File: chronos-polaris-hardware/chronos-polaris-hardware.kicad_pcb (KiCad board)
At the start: 2 copper layers, 65 parts, among them J1 Conn_01x03_Pin, J2 Conn_01x03_Pin, J3 Conn_01x03_Pin, J4 Conn_01x03_Pin, J5 Conn_01x03_Pin, J6 Conn_01x04, J7 Conn_01x04, J8 Conn_01x02, J9 691417320006S, Q1 US6K4TR, U1 TLV62130RGTR, U10 MSK12C02-HB, U11 TPS62172DSGR, U14 FC-B1010RGBT-HG, U2 ESP32-S2-SOLO-2-N4, U3 BMI088, U4 TYPE-C_14PLC-H10_0, U5 TF_PUSH, U6 TPS629206DRLR, U9 BMP280

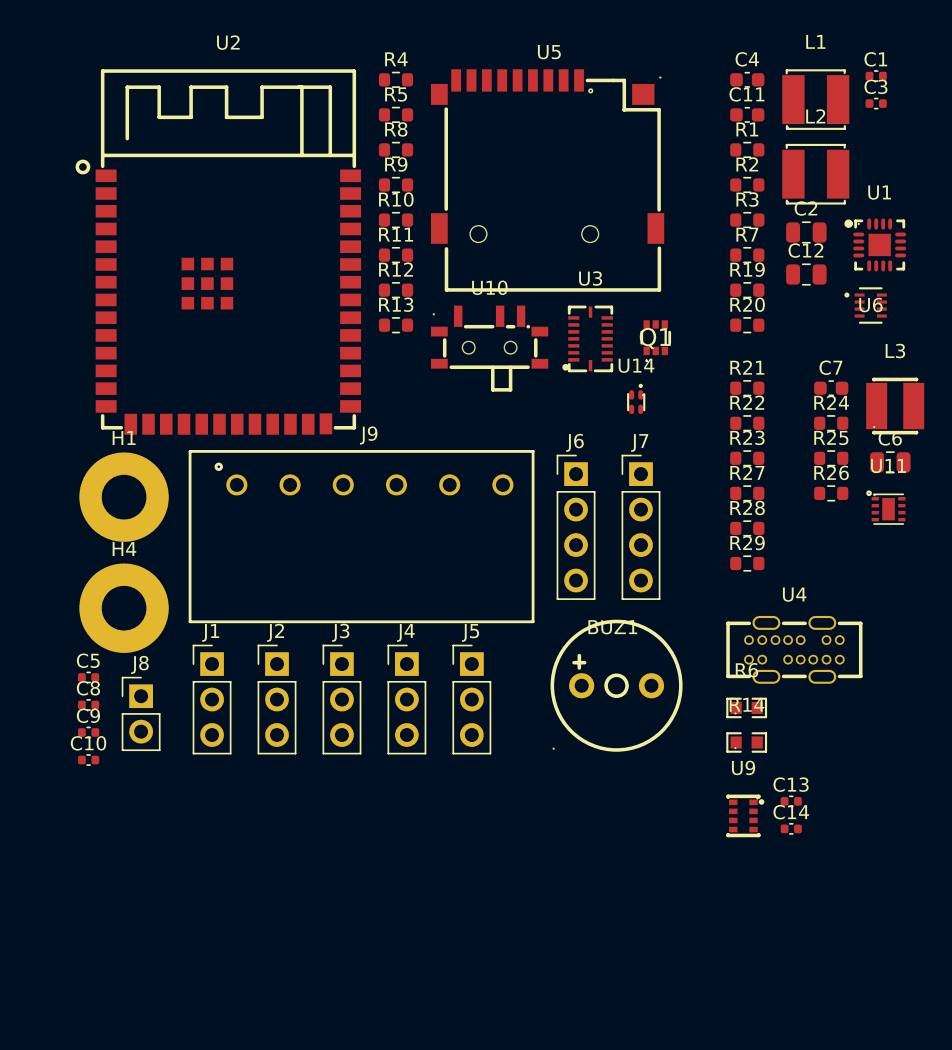
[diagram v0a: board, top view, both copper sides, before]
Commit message: pcb revert
a
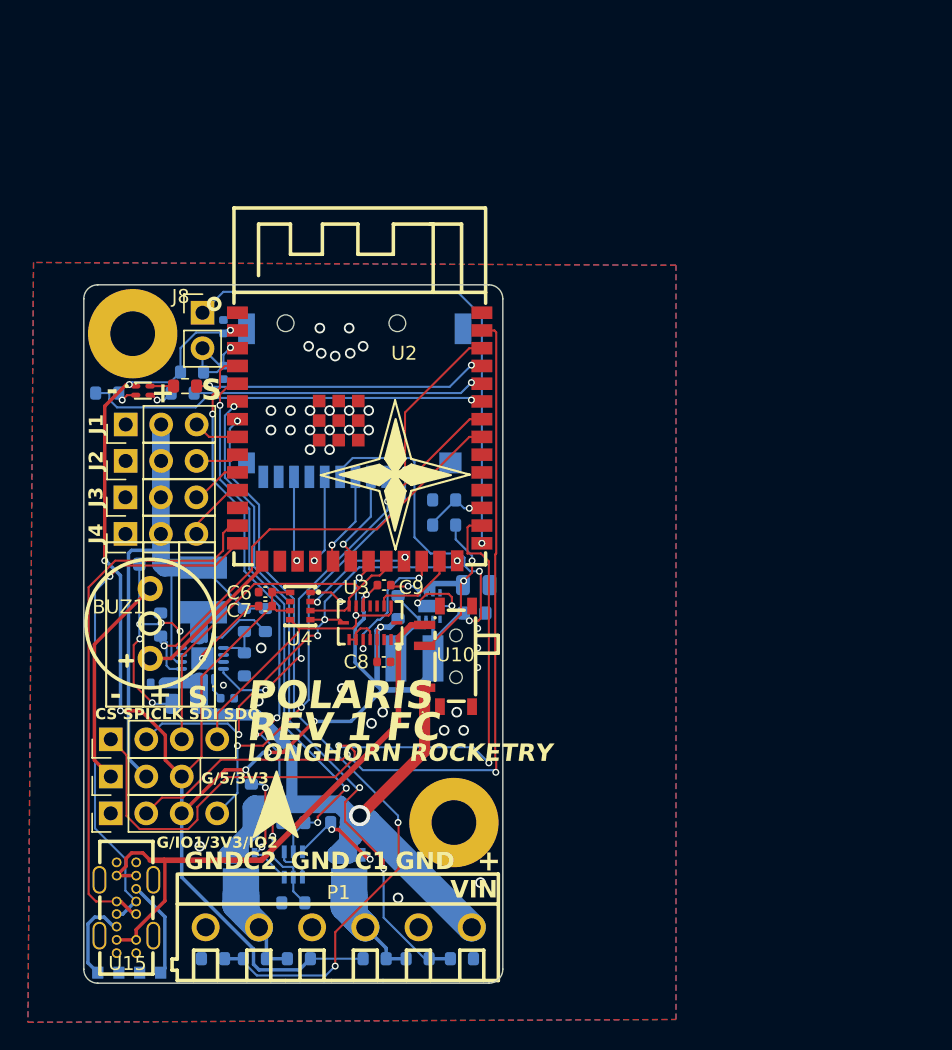
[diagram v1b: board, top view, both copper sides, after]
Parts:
- removed C13, C14: 100nF, Capacitor_SMD:C_0402_1005Metric
- removed J9: 691417320006S, polaris-fp:691417320006S
- removed L3: 2.2uH, polaris-fp:IND-SMD_L3.0-W3.0
- removed Q1: US6K4TR, KiCad:US6K4TR
- removed R24, R28: 30k, Resistor_SMD:R_0603_1608Metric
- removed R25, R27, R29: 10k, Resistor_SMD:R_0603_1608Metric
- removed R26: 100k, Resistor_SMD:R_0603_1608Metric
- removed U11: TPS62172DSGR, polaris-fp:WSON-8_L2.0-W2.0-P0.50-TL-EP
- removed U9: BMP280, polaris-fp:LGA-8_L2.5-W2.0-P0.65_AMP6127
- added P1: WJ124-3_81-6P, polaris-fp:CONN-TH_6P-P3.81_WJ124-3.81-6P, F.Cu at (118.2, 146.0)
- added R15: 10k, Resistor_SMD:R_0603_1608Metric, B.Cu at (127.1, 148.2)
- added R16: 10k, Resistor_SMD:R_0603_1608Metric, B.Cu at (115.4, 148.2)
- added R17: 30k, Resistor_SMD:R_0603_1608Metric, B.Cu at (112.2, 148.2)
- added R18: 10k, Resistor_SMD:R_0603_1608Metric, B.Cu at (109.2, 148.2)
- added U12: AP20P30Q, polaris-fp:DFN-8_L3.3-W3.0-P0.65-LS3.3-BL-EP, B.Cu at (119.0, 142.2)
- added U15: TYPE-C_14PLC-H10_0, polaris-fp:USB-C-TH_SHOUHAN_TYPE-C-14PLC-H10.0, F.Cu at (103.0, 144.6)
- added U7: AP20P30Q, polaris-fp:DFN-8_L3.3-W3.0-P0.65-LS3.3-BL-EP, B.Cu at (111.2, 142.2)
- added U8: 2N7002KDW_72K, polaris-fp:SOT-363_L2.1-W1.3-P0.65-LS2.3-BL, B.Cu at (115.0, 141.5)
- C1: value 100nF -> 22uF; footprint Capacitor_SMD:C_0402_1005Metric -> Capacitor_SMD:C_0603_1608Metric; moved to B.Cu
- C10, C2, C5, L2, R10, R21, R22, R23, R4, R5, R8, R9, U5: moved to B.Cu
- C11: value 22uF -> 3.3nF; footprint Capacitor_SMD:C_0603_1608Metric -> Capacitor_SMD:C_0402_1005Metric; moved to B.Cu
- C12: value 4.7uF -> 100nF; footprint Capacitor_SMD:C_0805_2012Metric -> Capacitor_SMD:C_0402_1005Metric; moved to B.Cu
- C3: value 3.3nF -> 22uF; footprint Capacitor_SMD:C_0402_1005Metric -> Capacitor_SMD:C_0603_1608Metric; moved to B.Cu
- C4: value 22uF -> 10uF; footprint Capacitor_SMD:C_0603_1608Metric -> Capacitor_SMD:C_0805_2012Metric; moved to B.Cu
- C6: value 10uF -> 100nF; footprint Capacitor_SMD:C_0805_2012Metric -> Capacitor_SMD:C_0402_1005Metric
- C7: value 22uF -> 100nF; footprint Capacitor_SMD:C_0603_1608Metric -> Capacitor_SMD:C_0402_1005Metric
- L1: footprint polaris-fp:IND-SMD_L4.0-W4.0 -> polaris-fp:IND-SMD_L3.0-W3.0; moved to B.Cu
- R1: value 10k -> 100k; moved to B.Cu
- R12, R13: value ? -> 0603WAF5101T5E; footprint Resistor_SMD:R_0603_1608Metric -> polaris-fp:R0603; moved to B.Cu
- R14: value 0603WAF5101T5E -> 30k; footprint polaris-fp:R0603 -> Resistor_SMD:R_0603_1608Metric; moved to B.Cu
- R19: value 30k -> 100k; moved to B.Cu
- R2: value 240k -> 10k; moved to B.Cu
- R20: value 100k -> 160k; moved to B.Cu
- R3: value 27.4k -> 10k; moved to B.Cu
- R6: value 0603WAF5101T5E -> 10k; footprint polaris-fp:R0603 -> Resistor_SMD:R_0603_1608Metric; moved to B.Cu
- R7: value 160k -> 30k; moved to B.Cu
- U1: value TLV62130RGTR -> TPS62172DSGR; footprint polaris-fp:QFN-16_L3.0-W3.0-P0.50-TL-EP -> polaris-fp:WSON-8_L2.0-W2.0-P0.50-TL-EP; moved to B.Cu
- U4: value TYPE-C_14PLC-H10_0 -> BMP280; footprint polaris-fp:USB-C-TH_SHOUHAN_TYPE-C-14PLC-H10.0 -> polaris-fp:LGA-8_L2.5-W2.0-P0.65_AMP6127
- U6: value TPS629206DRLR -> TLV62130RGTR; footprint footprints:SOT5X3-8_DRL_TEX -> polaris-fp:QFN-16_L3.0-W3.0-P0.50-TL-EP; moved to B.Cu
- moved C3 61.6 mm to (104.8, 120.0), turned to 180 degrees
- moved C4 60.1 mm to (107.3, 130.0), turned to 180 degrees
- moved R5 56.9 mm to (115.0, 144.2)
- moved R2 56.3 mm to (112.0, 136.6), turned to 90 degrees
- moved C11 55.9 mm to (110.3, 129.6), turned to 180 degrees
- moved C12 54.9 mm to (105.3, 128.5)
- moved U6 54.1 mm to (108.5, 126.8), turned to -90 degrees
- moved R4 53.7 mm to (115.0, 138.5), turned to 180 degrees
- moved L2 53.0 mm to (108.5, 121.8), turned to -90 degrees
- moved R12 53.0 mm to (101.8, 149.2), turned to 180 degrees
- moved R3 52.0 mm to (118.5, 138.5), turned to 180 degrees
- moved R13 49.6 mm to (104.8, 149.2)
- moved L1 49.3 mm to (123.7, 126.8), turned to 180 degrees
- moved C1 48.0 mm to (128.0, 123.5)
- moved R7 46.4 mm to (111.5, 127.2), turned to -90 degrees
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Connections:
- C1 pad 1: GND -> 3.3V
- C1 pad 2: /BAT+ -> GND
- C11 pad 2: 5V -> Net-(U6-SS/TR)
- C12 pad 1: VIN -> GND
- C12 pad 2: GND -> /BAT+
- C2 pad 1: /BAT+ -> VIN
- C3 pad 1: GND -> 5V
- C3 pad 2: Net-(U1-SS/TR) -> GND
- C4 pad 1: 5V -> /BAT+
- C6 pad 1: VIN -> 3.3V
- L1 pad 1: 5V -> Net-(U1-SW)
- L1 pad 2: Net-(L1-Pad2) -> 3.3V
- L2 pad 2: Net-(U6-SW) -> Net-(L2-Pad2)
- R1 pad 1: GND -> 3.3V
- R1 pad 2: Net-(U1-EN) -> Net-(U1-PG)
- R12 pad 1: /BAT+ -> GND
- R12 pad 2: /MAIN V+ -> Net-(U15-CC1)
- R13 pad 1: /BAT+ -> GND
- R13 pad 2: /DROGUE V+ -> Net-(U15-CC2)
- R14 pad 1: GND -> /MAIN V+
- R14 pad 2: Net-(U4-CC1) -> /MAIN DETECT
- R19 pad 1: Net-(U1-FB) -> Net-(U6-PG)
- R19 pad 2: GND -> 5V
- R2 pad 1: GND -> /BAT+
- R2 pad 2: Net-(U6-FB/VSET) -> Net-(U7-G)
- R20 pad 1: Net-(U1-PG) -> 5V
- R20 pad 2: 5V -> Net-(U6-FB)
- R21 pad 1: 3.3V -> GND
- R21 pad 2: /Voltage Divider/MAIN V+ -> 5V_ENABLE
- R22 pad 1: /Voltage Divider/MAIN V+ -> VIN
- R22 pad 2: /MAIN DETECT -> VIN_1/4
- R23 pad 1: /MAIN DETECT -> VIN_1/4
- R3 pad 1: Net-(U6-MODE/S-CONF) -> /BAT+
- R3 pad 2: GND -> Net-(U12-G)
- R4 pad 1: GND -> /DROGUE CTRL
- R4 pad 2: Net-(Q1-TR2_G) -> GND
- R5 pad 2: Net-(Q1-TR1_G) -> /MAIN CTRL
- R6 pad 1: GND -> 3.3V
- R6 pad 2: Net-(U4-CC2) -> /MAIN V+
- R7 pad 1: 5V -> Net-(U6-FB)
- R7 pad 2: Net-(U1-FB) -> GND
- U1 pad 1: Net-(L1-Pad2) -> GND
- U1 pad 2: Net-(L1-Pad2) -> VIN
- U1 pad 3: Net-(L1-Pad2) -> VIN
- U1 pad 4: Net-(U1-PG) -> GND
- U1 pad 5: Net-(U1-FB) -> GND
- U1 pad 6: GND -> 3.3V
- U1 pad 7: GND -> Net-(U1-SW)
- U1 pad 8: 5V_5%BOOST -> Net-(U1-PG)
- U1 pad 9: Net-(U1-SS/TR) -> GND
- U2 pad 13: /TypeC/IO19 -> Net-(U2-IO19)
- U2 pad 14: /TypeC/IO20 -> Net-(U2-IO20)
- U2 pad 4: Net-(Q1-TR2_G) -> /MAIN CTRL
- U2 pad 5: Net-(Q1-TR1_G) -> /DROGUE CTRL
- U6 pad 1: Net-(U6-FB/VSET) -> Net-(L2-Pad2)
- U6 pad 2: unconnected-(U6-PG-Pad2) -> Net-(L2-Pad2)
- U6 pad 3: 5V -> Net-(L2-Pad2)
- U6 pad 4: Net-(U6-SW) -> Net-(U6-PG)
- U6 pad 5: GND -> Net-(U6-FB)
- U6 pad 6: VIN -> GND
- U6 pad 7: VIN -> GND
- U6 pad 8: Net-(U6-MODE/S-CONF) -> 5V_5%BOOST
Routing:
- net 3.3V: track 0.00 -> 153.2 mm, vias 0 -> 11
- net /BAT+: track 0.00 -> 68.8 mm, vias 0 -> 1
- net Net-(J6-Pin_2): track 0.00 -> 59.9 mm, vias 0 -> 2
- net Net-(J7-Pin_1): track 0.00 -> 57.5 mm, vias 0 -> 2
- net /DROGUE DETECT: track 0.00 -> 54.7 mm, vias 0 -> 3
- net GND: track 0.00 -> 52.7 mm, vias 0 -> 46
- net /MAIN DETECT: track 0.00 -> 48.3 mm, vias 0 -> 3
- net 5V: track 0.00 -> 46.3 mm
- net /MAIN CTRL: track 0.00 -> 45.0 mm, vias 0 -> 5
- net /USB_5V: track 0.00 -> 43.2 mm
- net Net-(J6-Pin_4): track 0.00 -> 42.7 mm, vias 0 -> 3
- net /DROGUE CTRL: track 0.00 -> 39.7 mm, vias 0 -> 3
- net Net-(U2-IO19): track 0.00 -> 38.5 mm
- net /GPIO0 (BOOTLOADER): track 0.00 -> 37.6 mm, vias 0 -> 1
- net Net-(U2-IO20): track 0.00 -> 36.8 mm, vias 0 -> 1
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- added copper zone on B.Cu, net GND
- added copper zone on F.Cu, net GND
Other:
- board outline added: 30 x 50 mm
- board text added: "+"
- board text added: "-"
- board text added: "3.5-13V"
- board text added: "3v3"
- board text added: "5v"
- board text added: "C1"
- board text added: "C2"
- board text added: "CHRONOS ROCKETRY"
- board text added: "CS SPICLK SDI SDO"
- board text added: "G/5/3V3"
- board text added: "G/IO1/3V3/IO2"
- board text added: "GND"
- board text added: "LONGHORN ROCKETRY"
- board text added: "POLARIS"
- board text added: "REV 1 FC"
- board text added: "S"
- board text added: "VIN"

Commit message: finnaly
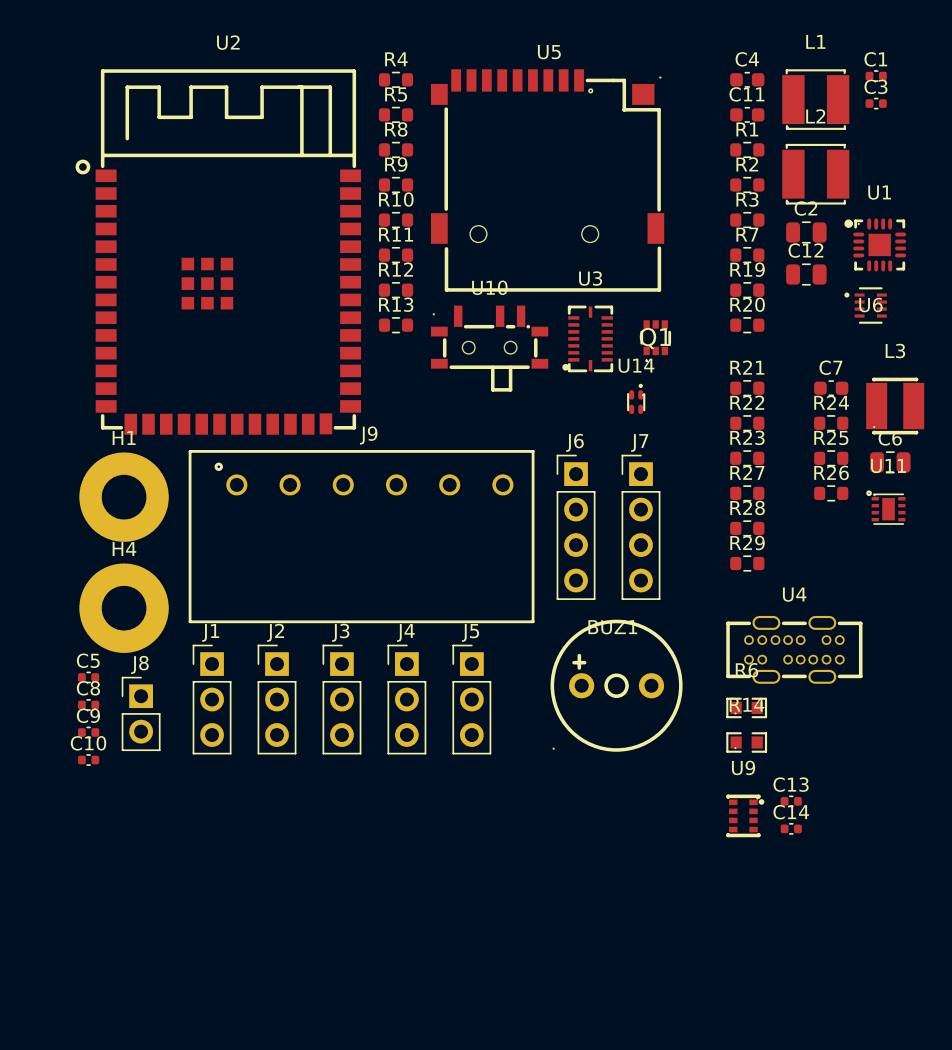
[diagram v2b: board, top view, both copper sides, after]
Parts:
- removed P1: WJ124-3_81-6P, polaris-fp:CONN-TH_6P-P3.81_WJ124-3.81-6P
- removed R15, R16, R18: 10k, Resistor_SMD:R_0603_1608Metric
- removed R17: 30k, Resistor_SMD:R_0603_1608Metric
- removed U12, U7: AP20P30Q, polaris-fp:DFN-8_L3.3-W3.0-P0.65-LS3.3-BL-EP
- removed U15: TYPE-C_14PLC-H10_0, polaris-fp:USB-C-TH_SHOUHAN_TYPE-C-14PLC-H10.0
- removed U8: 2N7002KDW_72K, polaris-fp:SOT-363_L2.1-W1.3-P0.65-LS2.3-BL
- added C13: 100nF, Capacitor_SMD:C_0402_1005Metric, F.Cu at (150.7, 137.0)
- added C14: 100nF, Capacitor_SMD:C_0402_1005Metric, F.Cu at (150.7, 139.0)
- added J9: 691417320006S, polaris-fp:691417320006S, F.Cu at (120.5, 114.3)
- added L3: 2.2uH, polaris-fp:IND-SMD_L3.0-W3.0, F.Cu at (158.1, 108.7)
- added Q1: US6K4TR, KiCad:US6K4TR, F.Cu at (140.9, 103.8)
- added R24: 30k, Resistor_SMD:R_0603_1608Metric, F.Cu at (153.5, 109.9)
- added R25: 10k, Resistor_SMD:R_0603_1608Metric, F.Cu at (153.5, 112.4)
- added R26: 100k, Resistor_SMD:R_0603_1608Metric, F.Cu at (153.5, 114.9)
- added R27: 10k, Resistor_SMD:R_0603_1608Metric, F.Cu at (147.5, 114.9)
- added R28: 30k, Resistor_SMD:R_0603_1608Metric, F.Cu at (147.5, 117.4)
- added R29: 10k, Resistor_SMD:R_0603_1608Metric, F.Cu at (147.5, 120.0)
- added U11: TPS62172DSGR, polaris-fp:WSON-8_L2.0-W2.0-P0.50-TL-EP, F.Cu at (157.6, 116.1)
- added U9: BMP280, polaris-fp:LGA-8_L2.5-W2.0-P0.65_AMP6127, F.Cu at (147.2, 138.0)
- C1: value 22uF -> 100nF; footprint Capacitor_SMD:C_0603_1608Metric -> Capacitor_SMD:C_0402_1005Metric; moved to F.Cu
- C10, C2, C5, L2, R10, R21, R22, R23, R4, R5, R8, R9, U5: moved to F.Cu
- C11: value 3.3nF -> 22uF; footprint Capacitor_SMD:C_0402_1005Metric -> Capacitor_SMD:C_0603_1608Metric; moved to F.Cu
- C12: value 100nF -> 4.7uF; footprint Capacitor_SMD:C_0402_1005Metric -> Capacitor_SMD:C_0805_2012Metric; moved to F.Cu
- C3: value 22uF -> 3.3nF; footprint Capacitor_SMD:C_0603_1608Metric -> Capacitor_SMD:C_0402_1005Metric; moved to F.Cu
- C4: value 10uF -> 22uF; footprint Capacitor_SMD:C_0805_2012Metric -> Capacitor_SMD:C_0603_1608Metric; moved to F.Cu
- C6: value 100nF -> 10uF; footprint Capacitor_SMD:C_0402_1005Metric -> Capacitor_SMD:C_0805_2012Metric
- C7: value 100nF -> 22uF; footprint Capacitor_SMD:C_0402_1005Metric -> Capacitor_SMD:C_0603_1608Metric
- L1: footprint polaris-fp:IND-SMD_L3.0-W3.0 -> polaris-fp:IND-SMD_L4.0-W4.0; moved to F.Cu
- R1: value 100k -> 10k; moved to F.Cu
- R12, R13: value 0603WAF5101T5E -> ?; footprint polaris-fp:R0603 -> Resistor_SMD:R_0603_1608Metric; moved to F.Cu
- R14: value 30k -> 0603WAF5101T5E; footprint Resistor_SMD:R_0603_1608Metric -> polaris-fp:R0603; moved to F.Cu
- R19: value 100k -> 30k; moved to F.Cu
- R2: value 10k -> 240k; moved to F.Cu
- R20: value 160k -> 100k; moved to F.Cu
- R3: value 10k -> 27.4k; moved to F.Cu
- R6: value 10k -> 0603WAF5101T5E; footprint Resistor_SMD:R_0603_1608Metric -> polaris-fp:R0603; moved to F.Cu
- R7: value 30k -> 160k; moved to F.Cu
- U1: value TPS62172DSGR -> TLV62130RGTR; footprint polaris-fp:WSON-8_L2.0-W2.0-P0.50-TL-EP -> polaris-fp:QFN-16_L3.0-W3.0-P0.50-TL-EP; moved to F.Cu
- U4: value BMP280 -> TYPE-C_14PLC-H10_0; footprint polaris-fp:LGA-8_L2.5-W2.0-P0.65_AMP6127 -> polaris-fp:USB-C-TH_SHOUHAN_TYPE-C-14PLC-H10.0
- U6: value TLV62130RGTR -> TPS629206DRLR; footprint polaris-fp:QFN-16_L3.0-W3.0-P0.50-TL-EP -> footprints:SOT5X3-8_DRL_TEX; moved to F.Cu
- moved C3 61.6 mm to (156.7, 87.0), turned to 0 degrees
- moved C4 60.1 mm to (147.5, 85.3), turned to 0 degrees
- moved R5 56.9 mm to (122.4, 87.8)
- moved R2 56.3 mm to (147.5, 92.9), turned to 0 degrees
- moved C11 55.9 mm to (147.5, 87.8), turned to 0 degrees
- moved C12 54.9 mm to (151.7, 99.3)
- moved U6 54.1 mm to (156.3, 101.5), turned to 0 degrees
- moved R4 53.7 mm to (122.4, 85.3), turned to 0 degrees
- moved L2 53.0 mm to (152.4, 92.1), turned to 0 degrees
- moved R12 53.0 mm to (122.4, 100.4), turned to 0 degrees
- moved R3 52.0 mm to (147.5, 95.4), turned to 0 degrees
- moved R13 49.6 mm to (122.4, 102.9)
- moved L1 49.3 mm to (152.4, 86.7), turned to 0 degrees
- moved C1 48.0 mm to (156.7, 85.1)
- moved R7 46.4 mm to (147.5, 97.9), turned to 0 degrees
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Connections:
- C1 pad 1: 3.3V -> GND
- C1 pad 2: GND -> /BAT+
- C11 pad 2: Net-(U6-SS/TR) -> 5V
- C12 pad 1: GND -> VIN
- C12 pad 2: /BAT+ -> GND
- C2 pad 1: VIN -> /BAT+
- C3 pad 1: 5V -> GND
- C3 pad 2: GND -> Net-(U1-SS/TR)
- C4 pad 1: /BAT+ -> 5V
- C6 pad 1: 3.3V -> VIN
- L1 pad 1: Net-(U1-SW) -> 5V
- L1 pad 2: 3.3V -> Net-(L1-Pad2)
- L2 pad 2: Net-(L2-Pad2) -> Net-(U6-SW)
- R1 pad 1: 3.3V -> GND
- R1 pad 2: Net-(U1-PG) -> Net-(U1-EN)
- R12 pad 1: GND -> /BAT+
- R12 pad 2: Net-(U15-CC1) -> /MAIN V+
- R13 pad 1: GND -> /BAT+
- R13 pad 2: Net-(U15-CC2) -> /DROGUE V+
- R14 pad 1: /MAIN V+ -> GND
- R14 pad 2: /MAIN DETECT -> Net-(U4-CC1)
- R19 pad 1: Net-(U6-PG) -> Net-(U1-FB)
- R19 pad 2: 5V -> GND
- R2 pad 1: /BAT+ -> GND
- R2 pad 2: Net-(U7-G) -> Net-(U6-FB/VSET)
- R20 pad 1: 5V -> Net-(U1-PG)
- R20 pad 2: Net-(U6-FB) -> 5V
- R21 pad 1: GND -> 3.3V
- R21 pad 2: 5V_ENABLE -> /Voltage Divider/MAIN V+
- R22 pad 1: VIN -> /Voltage Divider/MAIN V+
- R22 pad 2: VIN_1/4 -> /MAIN DETECT
- R23 pad 1: VIN_1/4 -> /MAIN DETECT
- R3 pad 1: /BAT+ -> Net-(U6-MODE/S-CONF)
- R3 pad 2: Net-(U12-G) -> GND
- R4 pad 1: /DROGUE CTRL -> GND
- R4 pad 2: GND -> Net-(Q1-TR2_G)
- R5 pad 2: /MAIN CTRL -> Net-(Q1-TR1_G)
- R6 pad 1: 3.3V -> GND
- R6 pad 2: /MAIN V+ -> Net-(U4-CC2)
- R7 pad 1: Net-(U6-FB) -> 5V
- R7 pad 2: GND -> Net-(U1-FB)
- U1 pad 1: GND -> Net-(L1-Pad2)
- U1 pad 2: VIN -> Net-(L1-Pad2)
- U1 pad 3: VIN -> Net-(L1-Pad2)
- U1 pad 4: GND -> Net-(U1-PG)
- U1 pad 5: GND -> Net-(U1-FB)
- U1 pad 6: 3.3V -> GND
- U1 pad 7: Net-(U1-SW) -> GND
- U1 pad 8: Net-(U1-PG) -> 5V_5%BOOST
- U1 pad 9: GND -> Net-(U1-SS/TR)
- U2 pad 13: Net-(U2-IO19) -> /TypeC/IO19
- U2 pad 14: Net-(U2-IO20) -> /TypeC/IO20
- U2 pad 4: /MAIN CTRL -> Net-(Q1-TR2_G)
- U2 pad 5: /DROGUE CTRL -> Net-(Q1-TR1_G)
- U6 pad 1: Net-(L2-Pad2) -> Net-(U6-FB/VSET)
- U6 pad 2: Net-(L2-Pad2) -> unconnected-(U6-PG-Pad2)
- U6 pad 3: Net-(L2-Pad2) -> 5V
- U6 pad 4: Net-(U6-PG) -> Net-(U6-SW)
- U6 pad 5: Net-(U6-FB) -> GND
- U6 pad 6: GND -> VIN
- U6 pad 7: GND -> VIN
- U6 pad 8: 5V_5%BOOST -> Net-(U6-MODE/S-CONF)
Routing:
- net 3.3V: track 153.2 -> 0.00 mm, vias 11 -> 0
- net /BAT+: track 68.8 -> 0.00 mm, vias 1 -> 0
- net Net-(J6-Pin_2): track 59.9 -> 0.00 mm, vias 2 -> 0
- net Net-(J7-Pin_1): track 57.5 -> 0.00 mm, vias 2 -> 0
- net /DROGUE DETECT: track 54.7 -> 0.00 mm, vias 3 -> 0
- net GND: track 52.7 -> 0.00 mm, vias 46 -> 0
- net /MAIN DETECT: track 48.3 -> 0.00 mm, vias 3 -> 0
- net 5V: track 46.3 -> 0.00 mm
- net /MAIN CTRL: track 45.0 -> 0.00 mm, vias 5 -> 0
- net /USB_5V: track 43.2 -> 0.00 mm
- net Net-(J6-Pin_4): track 42.7 -> 0.00 mm, vias 3 -> 0
- net /DROGUE CTRL: track 39.7 -> 0.00 mm, vias 3 -> 0
- net Net-(U2-IO19): track 38.5 -> 0.00 mm
- net /GPIO0 (BOOTLOADER): track 37.6 -> 0.00 mm, vias 1 -> 0
- net Net-(U2-IO20): track 36.8 -> 0.00 mm, vias 1 -> 0
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- removed copper zone on B.Cu, net GND
- removed copper zone on F.Cu, net GND
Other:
- board outline removed
- board text removed: "+"
- board text removed: "-"
- board text removed: "3.5-13V"
- board text removed: "3v3"
- board text removed: "5v"
- board text removed: "C1"
- board text removed: "C2"
- board text removed: "CHRONOS ROCKETRY"
- board text removed: "CS SPICLK SDI SDO"
- board text removed: "G/5/3V3"
- board text removed: "G/IO1/3V3/IO2"
- board text removed: "GND"
- board text removed: "LONGHORN ROCKETRY"
- board text removed: "POLARIS"
- board text removed: "REV 1 FC"
- board text removed: "S"
- board text removed: "VIN"
